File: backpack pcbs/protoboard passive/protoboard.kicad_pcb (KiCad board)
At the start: 2 copper layers, 30 x 22.5 mm, 73 parts, among them J1 Conn_01x05_Male, J2 Conn_01x08_Female, J3 Conn_01x08_Female

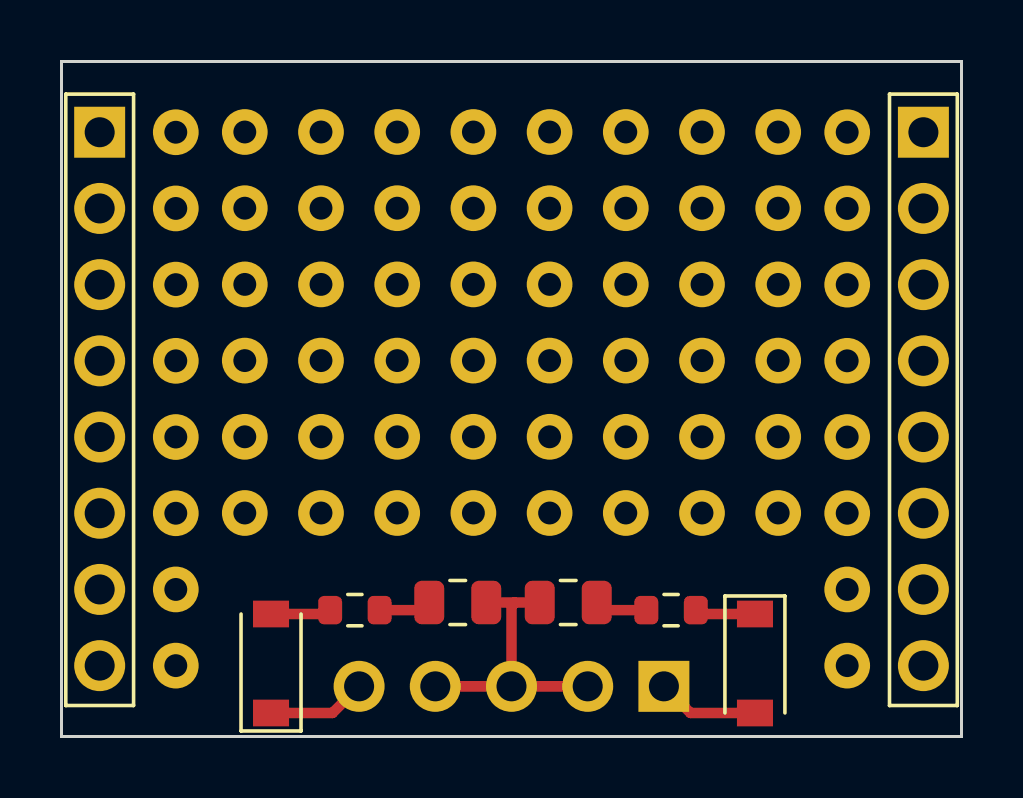
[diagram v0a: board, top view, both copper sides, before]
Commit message: kicad save, add panel, add passive protoboard, gerbers
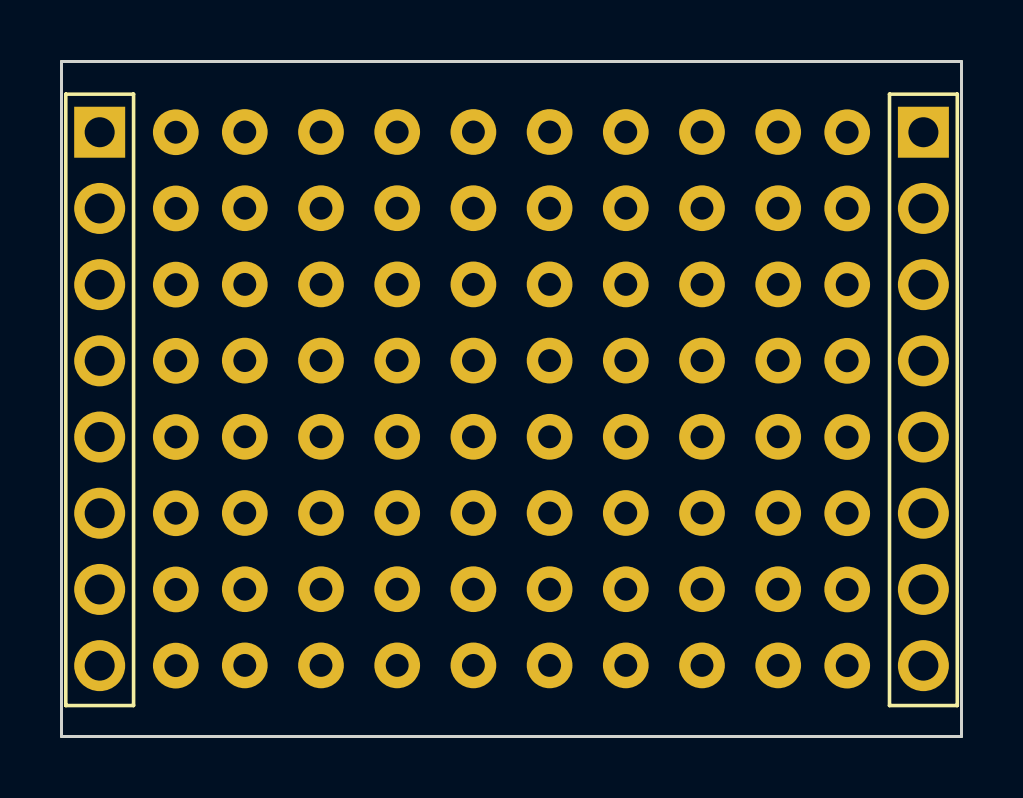
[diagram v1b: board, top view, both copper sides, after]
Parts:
- removed C1, C2: 10uF, Capacitor_SMD:C_0805_2012Metric
- removed D1, D2: 1N5817, Diode_SMD:D_SOD-123
- removed FB1, FB2: FerriteBead_Small, Resistor_SMD:R_0603_1608Metric
- removed J1: Conn_01x05_Male, Connector_PinHeader_2.54mm:PinHeader_1x05_P2.54mm_Vertical
- added 59: , , F.Cu at (6.11, 17.6)
- added 60: , , F.Cu at (8.65, 17.6)
- added 61: , , F.Cu at (11.2, 17.6)
- added 62: , , F.Cu at (13.7, 17.6)
- added 63: , , F.Cu at (16.3, 17.6)
- added 64: , , F.Cu at (18.8, 17.6)
- added 65: , , F.Cu at (21.4, 17.6)
- added 66: , , F.Cu at (23.9, 17.6)
- added 67: , , F.Cu at (6.11, 20.1)
- added 68: , , F.Cu at (8.65, 20.1)
- added 69: , , F.Cu at (11.2, 20.1)
- added 70: , , F.Cu at (13.7, 20.1)
- added 71: , , F.Cu at (16.3, 20.1)
- added 72: , , F.Cu at (18.8, 20.1)
- added 73: , , F.Cu at (21.4, 20.1)
- added 74: , , F.Cu at (23.9, 20.1)
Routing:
- net GND: track 9.70 -> 0.00 mm
- net Net-(D1-Pad2): track 3.40 -> 0.00 mm
- net Net-(D2-Pad1): track 3.30 -> 0.00 mm
- net Net-(D1-Pad1): track 2.02 -> 0.00 mm
- net Net-(D2-Pad2): track 2.02 -> 0.00 mm
- net -12V: track 1.76 -> 0.00 mm
- net +12V: track 1.76 -> 0.00 mm
